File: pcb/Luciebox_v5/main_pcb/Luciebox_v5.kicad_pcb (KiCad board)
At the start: 2 copper layers, 78 x 90.5 mm, 65 parts, among them J1 USB_B_Mini, J2 USB_B_Mini, Q1 P-Channel MOSFET, Q2 NPN transistor, T1 terminal_8x1, T2 terminal_3x1, T4 terminal_8x1, T5 terminal_3x1, T6 terminal_8x1, T7 terminal_8x1, T8 terminal_8x1, U1 CA56-12SRWA, U2 8X8PADS, U3 ATmega328-PU, Y1 16MHz

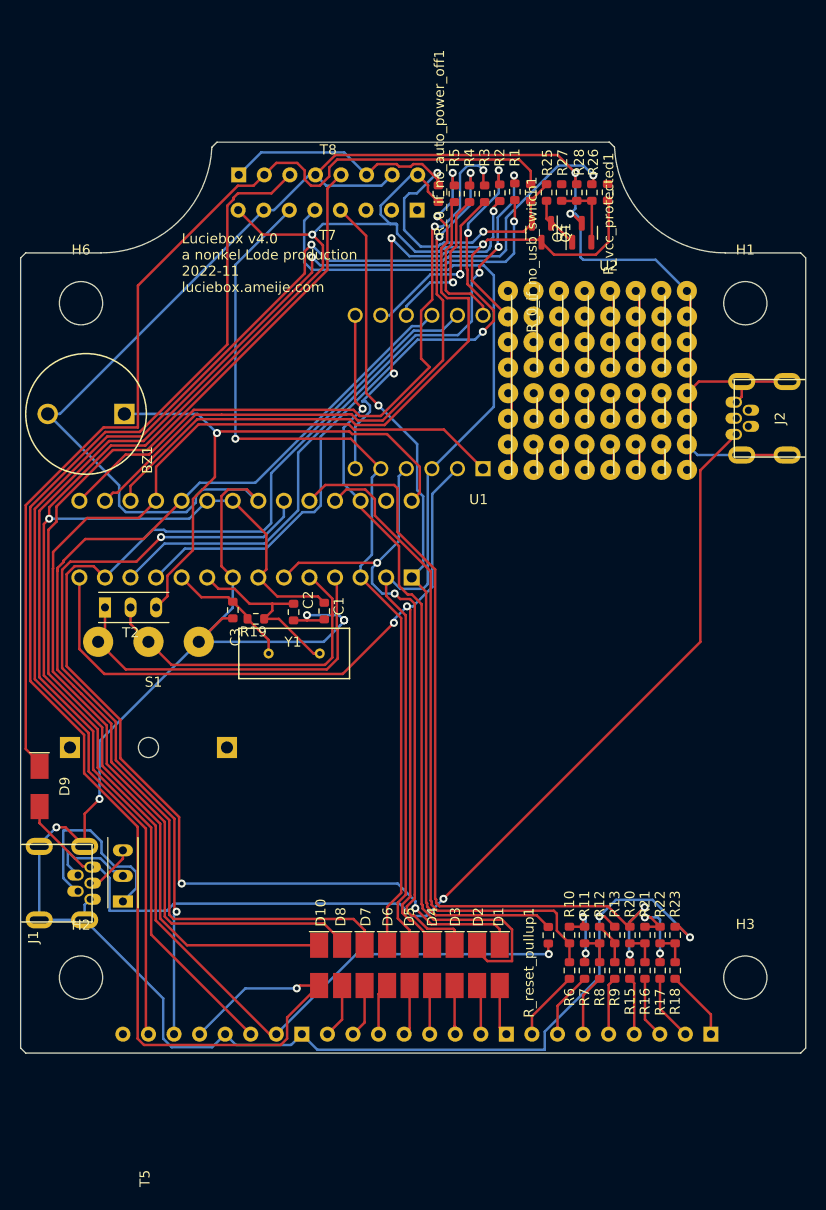
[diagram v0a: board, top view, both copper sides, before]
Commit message: Pcb V5
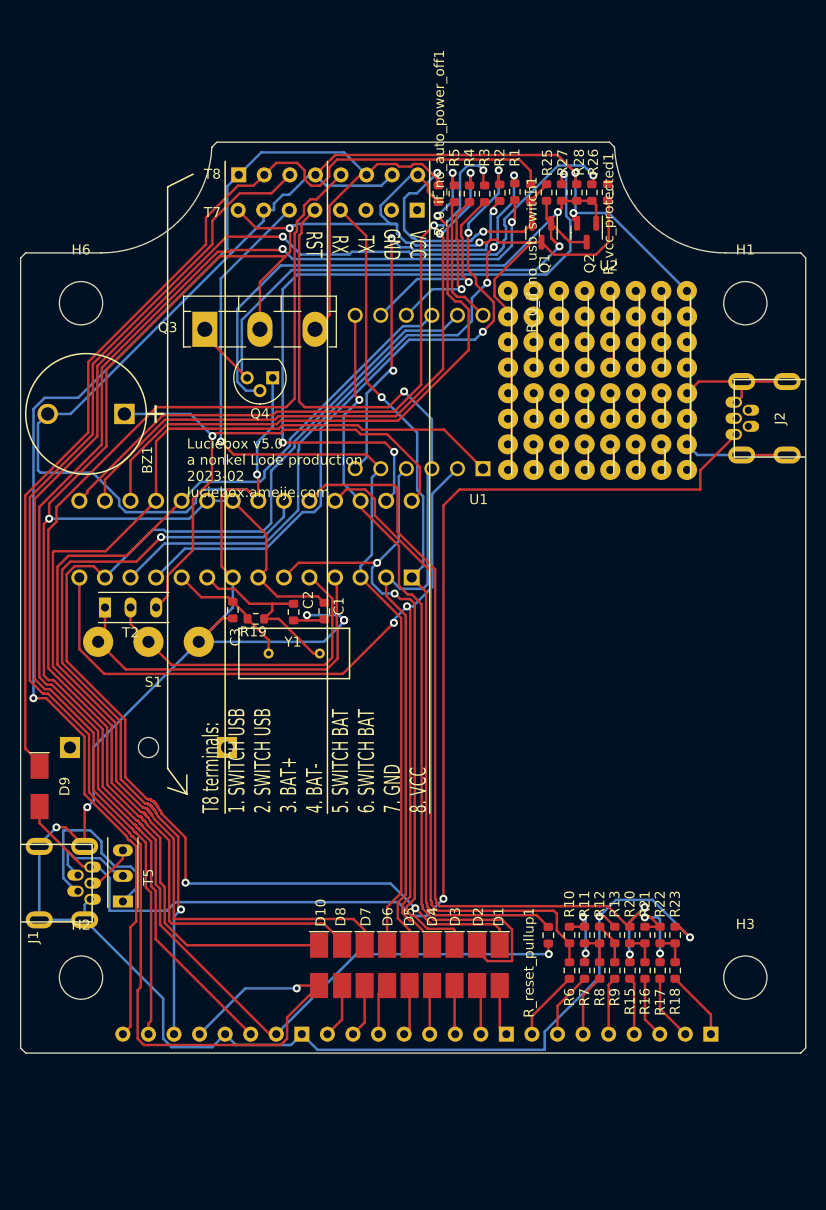
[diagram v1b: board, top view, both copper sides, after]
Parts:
- added Q3: P-Channel MOSFET_through hole, Package_TO_SOT_THT:TO-218-3_Vertical, F.Cu at (18.3, 18.6)
- added Q4: NPN_transistor_TO-92, Package_TO_SOT_THT:TO-92, F.Cu at (25.0, 23.4)
- moved Q2 0.49 mm to (56.2, 8.99), turned to -90 degrees
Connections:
- Q2 pad 1: Net-(Q1-Pad1) -> Net-(Q2-Pad1)
- Q2 pad 2: Net-(Q2-Pad2) -> GND
- Q2 pad 3: GND -> Net-(Q1-Pad1)
- R26 pad 1: Net-(Q2-Pad2) -> Net-(Q2-Pad1)
- R27 pad 1: Net-(Q2-Pad2) -> Net-(Q2-Pad1)
- R28 pad 2: Net-(Q2-Pad2) -> Net-(Q2-Pad1)
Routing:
- net /Vin: track 51.2 -> 170.0 mm, vias 2 -> 3
- net /A4(SDA): track 0.00 -> 71.0 mm, vias 0 -> 3
- net Net-(Q1-Pad1): track 5.30 -> 58.0 mm, vias 0 -> 1
- net Net-(Q2-Pad1): track 0.00 -> 52.4 mm, vias 0 -> 1
- net GND: track 344.4 -> 359.2 mm, vias 9 -> 10
- net Net-(D9-Pad2): track 107.0 -> 121.1 mm
- net VCC: track 252.2 -> 261.3 mm
- net /0(Rx): track 101.7 -> 94.4 mm, vias 0 -> 1
- net Net-(Q2-Pad2): track 7.15 -> 0.00 mm
- net Net-(D10-Pad1): track 109.4 -> 115.4 mm
- net Net-(R26-Pad2): track 132.3 -> 136.5 mm
- net Net-(R1-Pad1): track 125.4 -> 129.1 mm
- net /1(Tx): track 91.0 -> 93.2 mm
- net Net-(D9-Pad1): track 103.8 -> 101.9 mm
- net Net-(R3-Pad1): track 17.8 -> 19.6 mm, vias 2 -> 1
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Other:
- board text added: "12 Drawing 13 The void 14 Music 15 Media Player 16 Metronome 17 Sequencer 18 Notes 19 Composer 20 Noise 21 Hacker 22 Baby"
- board text added: "A Nonkel Lode Production | 2023"
- board text added: "B1 B2,3 B4 B5,6,7,8"
- board text added: "Button functions Control Button Options|Shift Start|Stop|Auto Action Buttons"
- board text added: "Buttons"
- board text added: "Control Power On Power Off App Select App Reset"
- board text added: "Luciebox v5.0 a nonkel Lode production 2023-02 luciebox.ameije.com"
- board text added: "T8 terminals: 1. SWITCH USB 2. SWITCH USB 3. BAT+ 4. BAT- 5. SWITCH BAT 6. SWITCH BAT 7. GND 8. VCC"
- board text added: "VCC GND TX RX RST"
- board text removed: "12 Drawing 13 Memory 14 Music 15 Media Player 16 Metronome 17 Sequencer 18 Notes 19 Composer 20 Noise 21 Hacker 22 Baby"
- board text removed: "A Nonkel Lode Production | 2022"
- board text removed: "B1 B2,B3 B4 B5,B6,B7,B8"
- board text removed: "Buttons Control Button Options|Shift Start|Stop|Auto Action Buttons"
- board text removed: "Control Box On Box Off App Select App Reset"
- board text removed: "Luciebox v4.0 a nonkel Lode production 2022-11 luciebox.ameije.com"
